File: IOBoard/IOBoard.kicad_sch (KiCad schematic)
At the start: 1 part, among them J1 Conn_02x20_Odd_Even

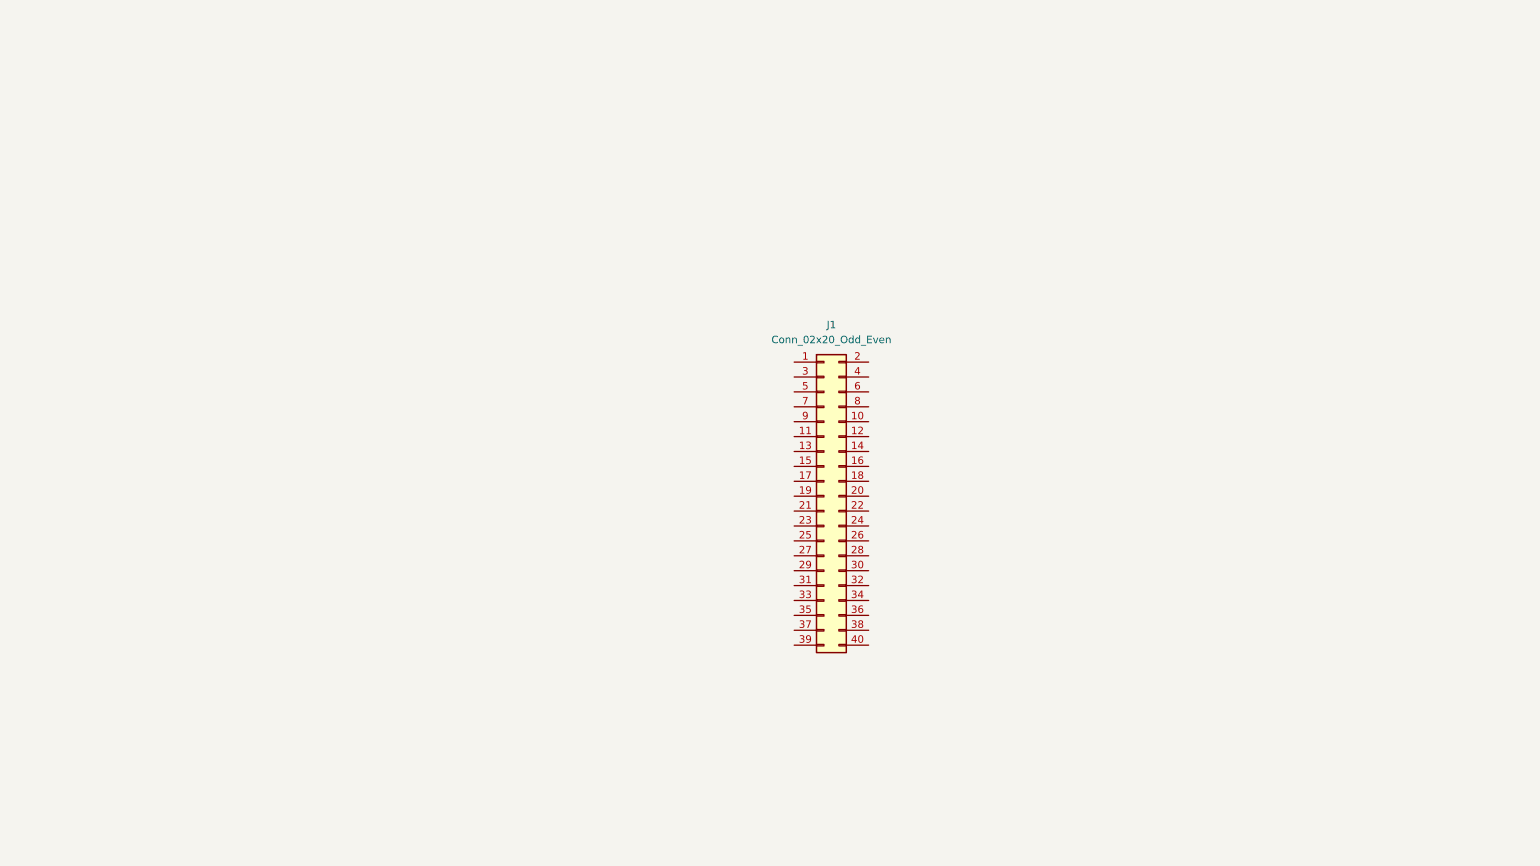
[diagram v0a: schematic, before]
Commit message: complete schematic for usb hub
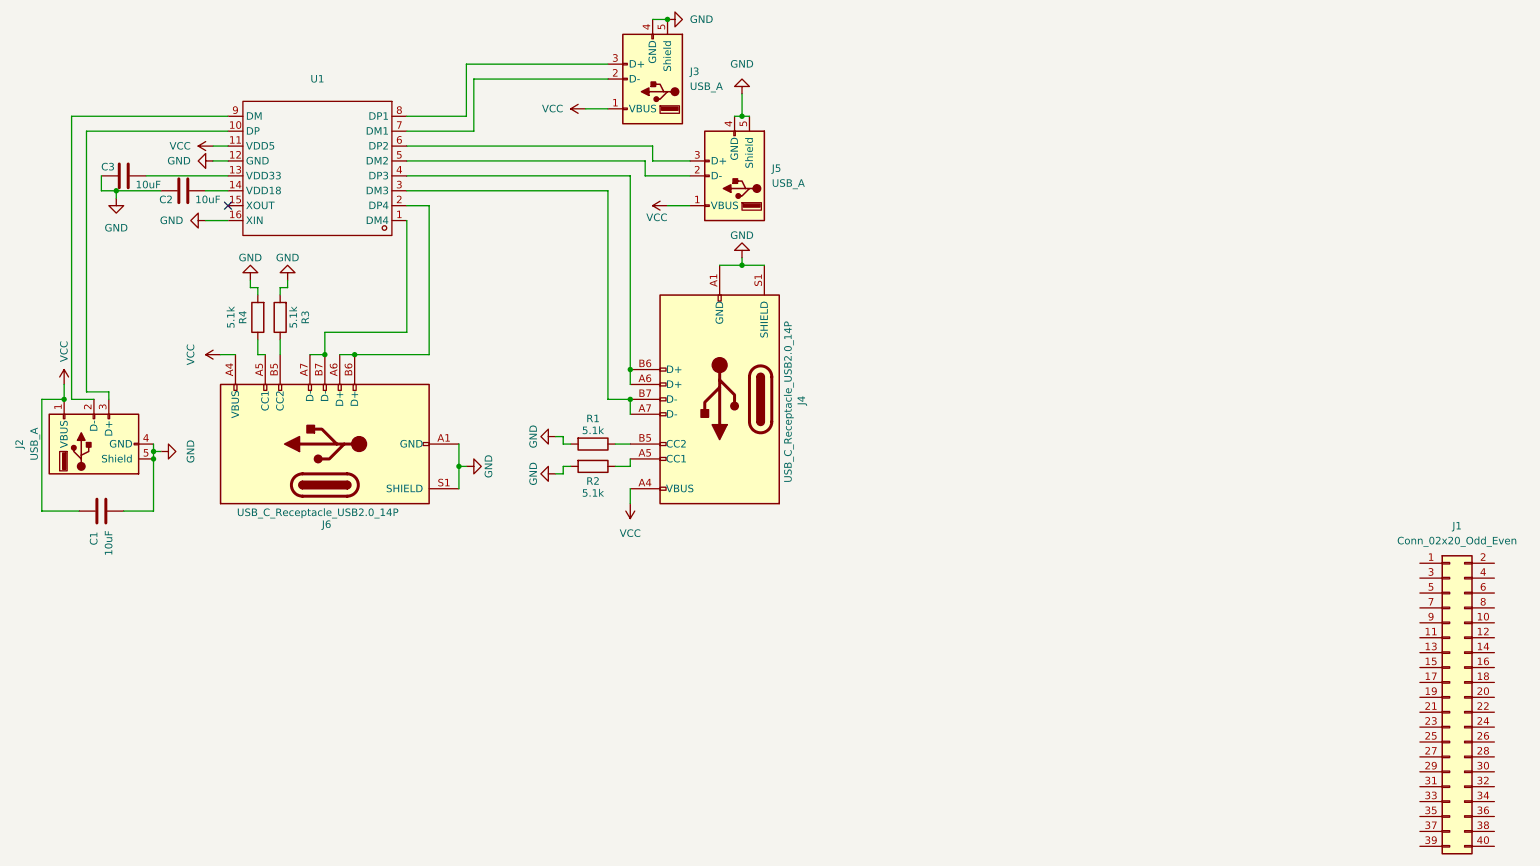
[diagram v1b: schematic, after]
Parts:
- added C1, C2, C3: 10uF, symbol Device:C
- added J2, J3, J5: USB_A, symbol Connector:USB_A
- added J4, J6: USB_C_Receptacle_USB2.0_14P, symbol Connector:USB_C_Receptacle_USB2.0_14P
- added R1, R2, R3, R4: 5.1k, symbol Device:R
- added U1: ~, SL2.1A:SOP-16_L10.0-W3.9-P1.27-LS6.0-BL, symbol SL2.1A:SL2.1A
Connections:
- new net: C3.2, U1.13 (VDD33)
- new net: J4.A5 (CC1), R2.1
- new net: J4.A6 (D+), J4.B6 (D+), U1.4 (DP3)
- new net: J4.A7 (D-), J4.B7 (D-), U1.3 (DM3)
- new net: J4.B5 (CC2), R1.1
- new net: J6.A5 (CC1), R4.1
- new net: J3.2 (D-), U1.7 (DM1)
- new net: J3.3 (D+), U1.8 (DP1)
- new net: J6.A6 (D+), J6.B6 (D+), U1.2 (DP4)
- new net: J6.A7 (D-), J6.B7 (D-), U1.1 (DM4)
- new net: J6.B5 (CC2), R3.1
- new net: J2.3 (D+), U1.10 (DP)
- new net: C2.2, U1.14 (VDD18)
- new net: J5.2 (D-), U1.5 (DM2)
- new net: J5.3 (D+), U1.6 (DP2)
- new net: J2.2 (D-), U1.9 (DM)
- new net GND: C1.2, C2.1, C3.1, J2.4 (GND), J2.5 (Shield), J3.4 (GND), J3.5 (Shield), J4.A1 (GND), J4.A12 (GND), J4.B1 (GND), J4.B12 (GND), J4.S1 (SHIELD), J5.4 (GND), J5.5 (Shield), J6.A1 (GND), J6.A12 (GND), J6.B1 (GND), J6.B12 (GND), J6.S1 (SHIELD), R1.2, R2.2, R3.2, R4.2, U1.12 (GND), U1.16 (XIN)
- new net VCC: C1.1, J2.1 (VBUS), J3.1 (VBUS), J4.A4 (VBUS), J4.A9 (VBUS), J4.B4 (VBUS), J4.B9 (VBUS), J5.1 (VBUS), J6.A4 (VBUS), J6.A9 (VBUS), J6.B4 (VBUS), J6.B9 (VBUS), U1.11 (VDD5)
- no-connect marks 0 -> 1
